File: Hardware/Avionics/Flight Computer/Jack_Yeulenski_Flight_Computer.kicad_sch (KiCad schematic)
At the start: 20 parts, among them J1 SW, J2 BAT, J3 UART Radio Connector, J4 I2C GPS Connector

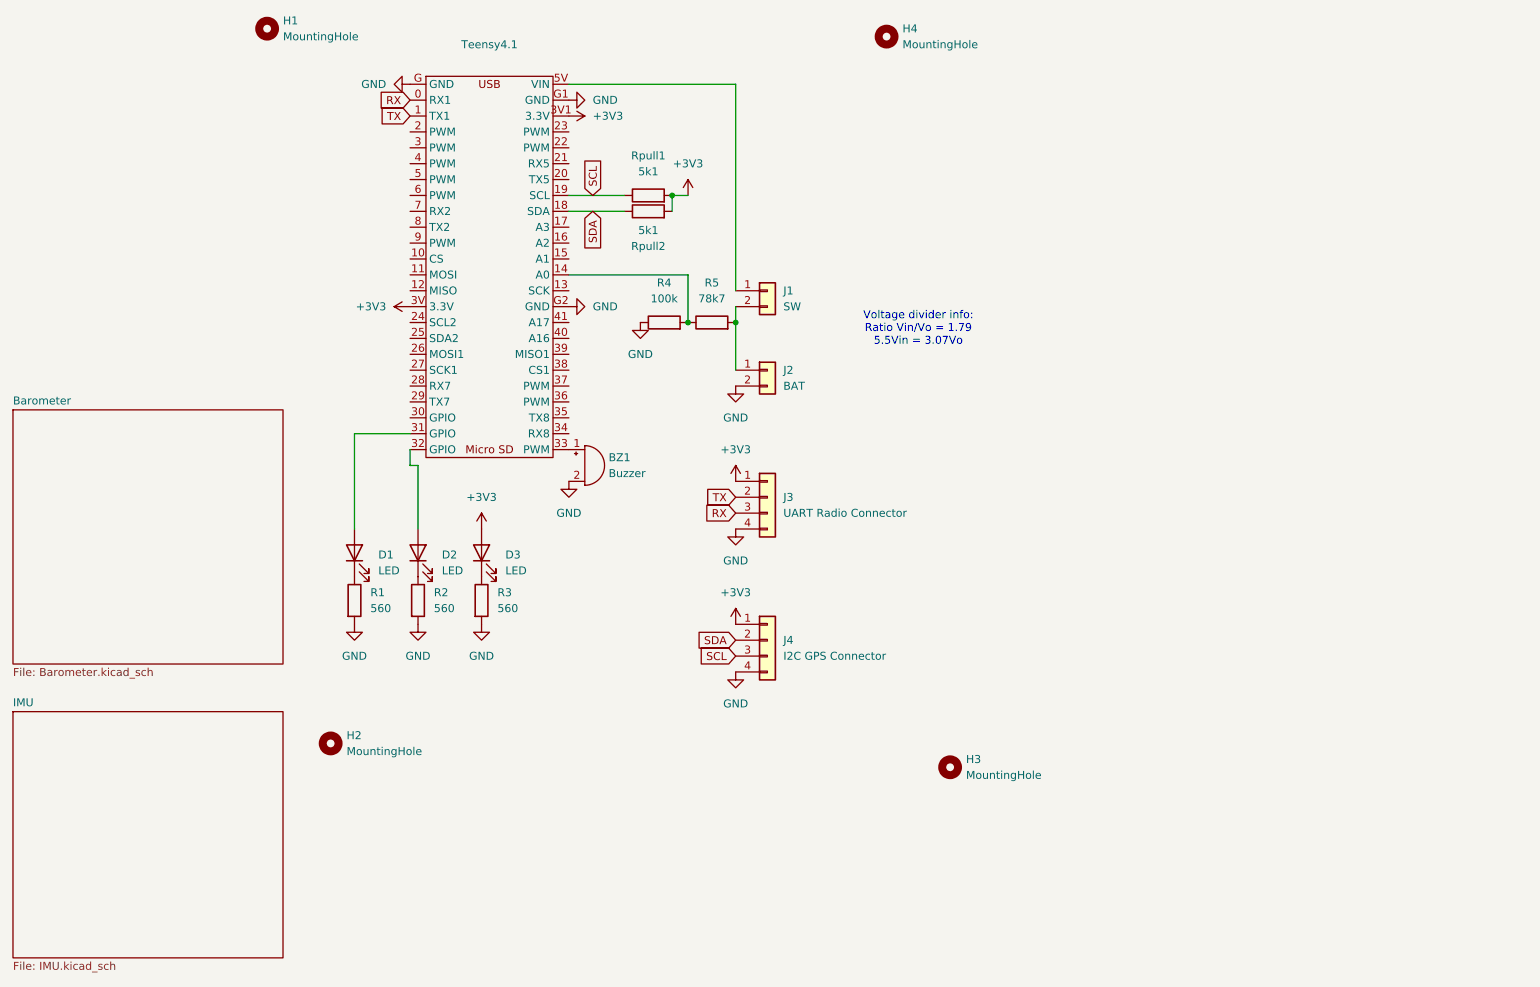
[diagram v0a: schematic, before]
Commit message: PCB updates
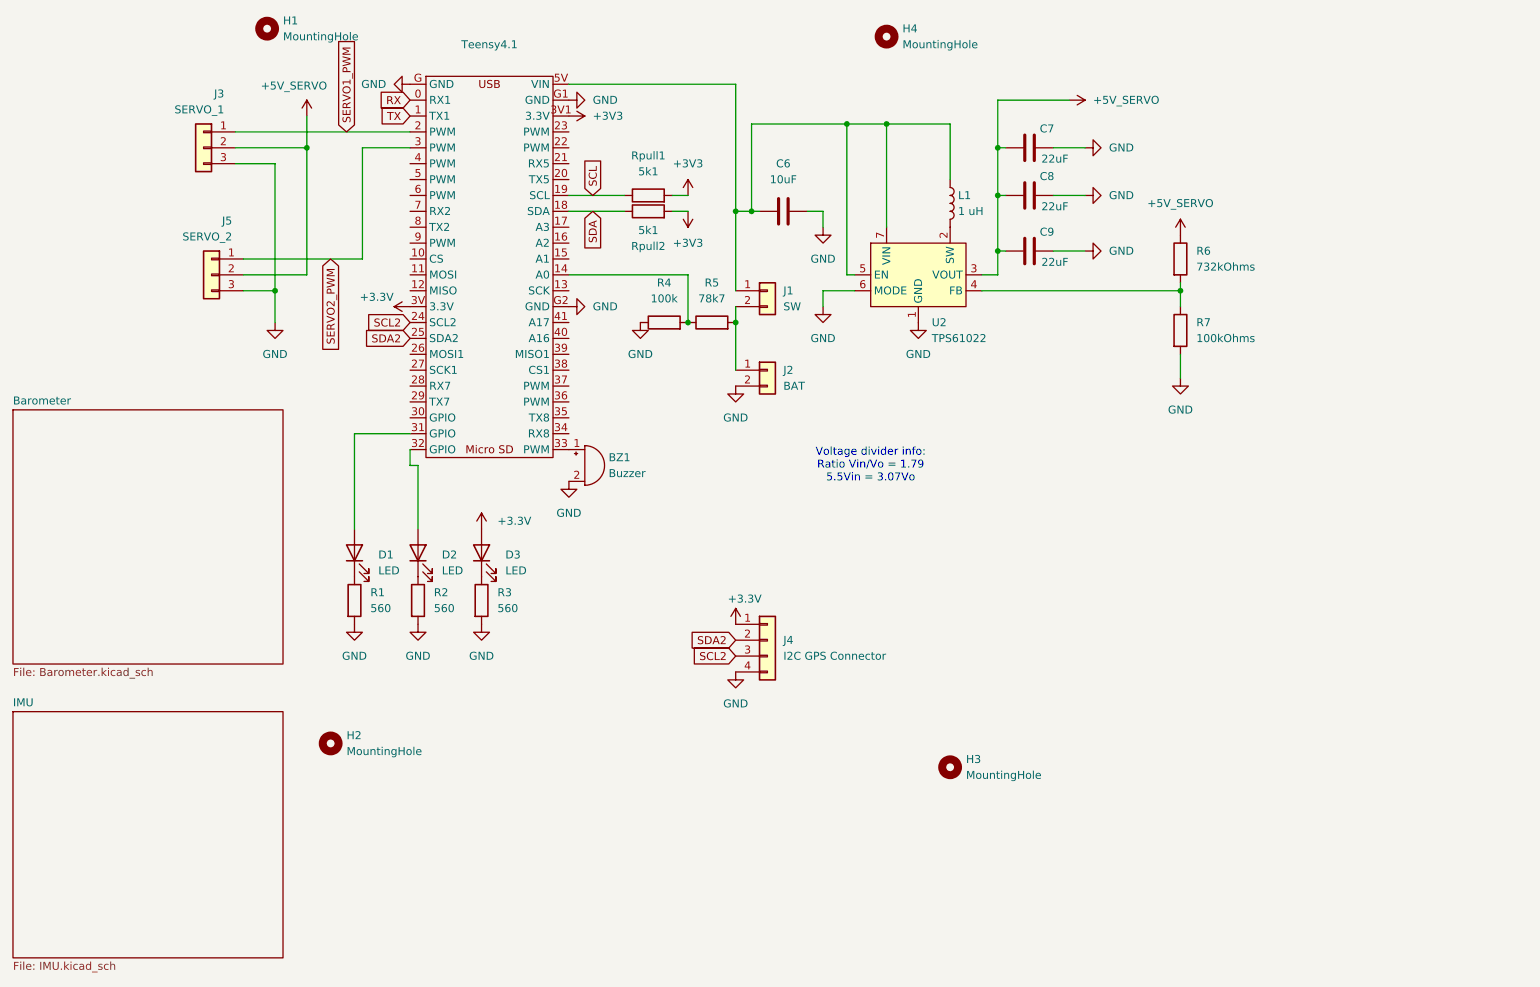
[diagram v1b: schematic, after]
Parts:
- removed J3: UART Radio Connector, Connector_JST:JST_XH_S4B-XH-A_1x04_P2.50mm_Horizontal, symbol Connector_Generic:Conn_01x04
- added C6: 10uF, Capacitor_SMD:C_0805_2012Metric, symbol Device:C
- added C7, C8, C9: 22uF, Capacitor_SMD:C_0805_2012Metric, symbol Device:C
- added J3: SERVO_1, Connector_PinHeader_2.54mm:PinHeader_1x03_P2.54mm_Vertical, symbol Connector_Generic:Conn_01x03
- added J5: SERVO_2, Connector_PinHeader_2.54mm:PinHeader_1x03_P2.54mm_Vertical, symbol Connector_Generic:Conn_01x03
- added L1: 1 uH, Inductor_SMD:L_Coilcraft_XAL7030-102, symbol Device:L
- added R6: 732kOhms, Resistor_SMD:R_0603_1608Metric, symbol Device:R
- added R7: 100kOhms, Resistor_SMD:R_0603_1608Metric, symbol Device:R
- added U2: TPS61022, Package_DFN_QFN:Texas_RWU0007A_VQFN-7_2x2mm_P0.5mm, symbol Converter_DCDC:TPS61022
- Teensy4.1: value ~ -> (none)
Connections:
- net +3V3: no longer D3.2 (A), J4.1 (Pin_1), Teensy4.1.3V (3.3V)
- net GND: now also C6.2, C7.2, C8.2, C9.2, J3.3 (GND), J5.3 (GND), R7.2, U2.1 (GND), U2.6 (MODE)
- net SCL: no longer J4.3 (Pin_3)
- net SDA: no longer J4.2 (Pin_2)
- net SERVO1_PWM: now reaches Teensy4.1.2 (PWM)
- net SERVO1_PWM: now also J3.1 (SERVO_PWM)
- net SCL2: now reaches Teensy4.1.24 (SCL2)
- net SCL2: now also J4.3 (Pin_3)
- net SDA2: now reaches Teensy4.1.25 (SDA2)
- net SDA2: now also J4.2 (Pin_2)
- net SERVO2_PWM: now reaches Teensy4.1.3 (PWM)
- net SERVO2_PWM: now also J5.1 (SERVO_PWM)
- net at J1.1 (Pin_1), Teensy4.1.5V (VIN): now also C6.1, L1.1, U2.5 (EN), U2.7 (VIN)
- new net: L1.2, U2.2 (SW)
- new net: R6.2, R7.1, U2.4 (FB)
- new net +3.3V: D3.2 (A), J4.1 (Pin_1), Teensy4.1.3V (3.3V)
- new net +5V_SERVO: C7.1, C8.1, C9.1, J3.2 (+5V), J5.2 (+5V), R6.1, U2.3 (VOUT)

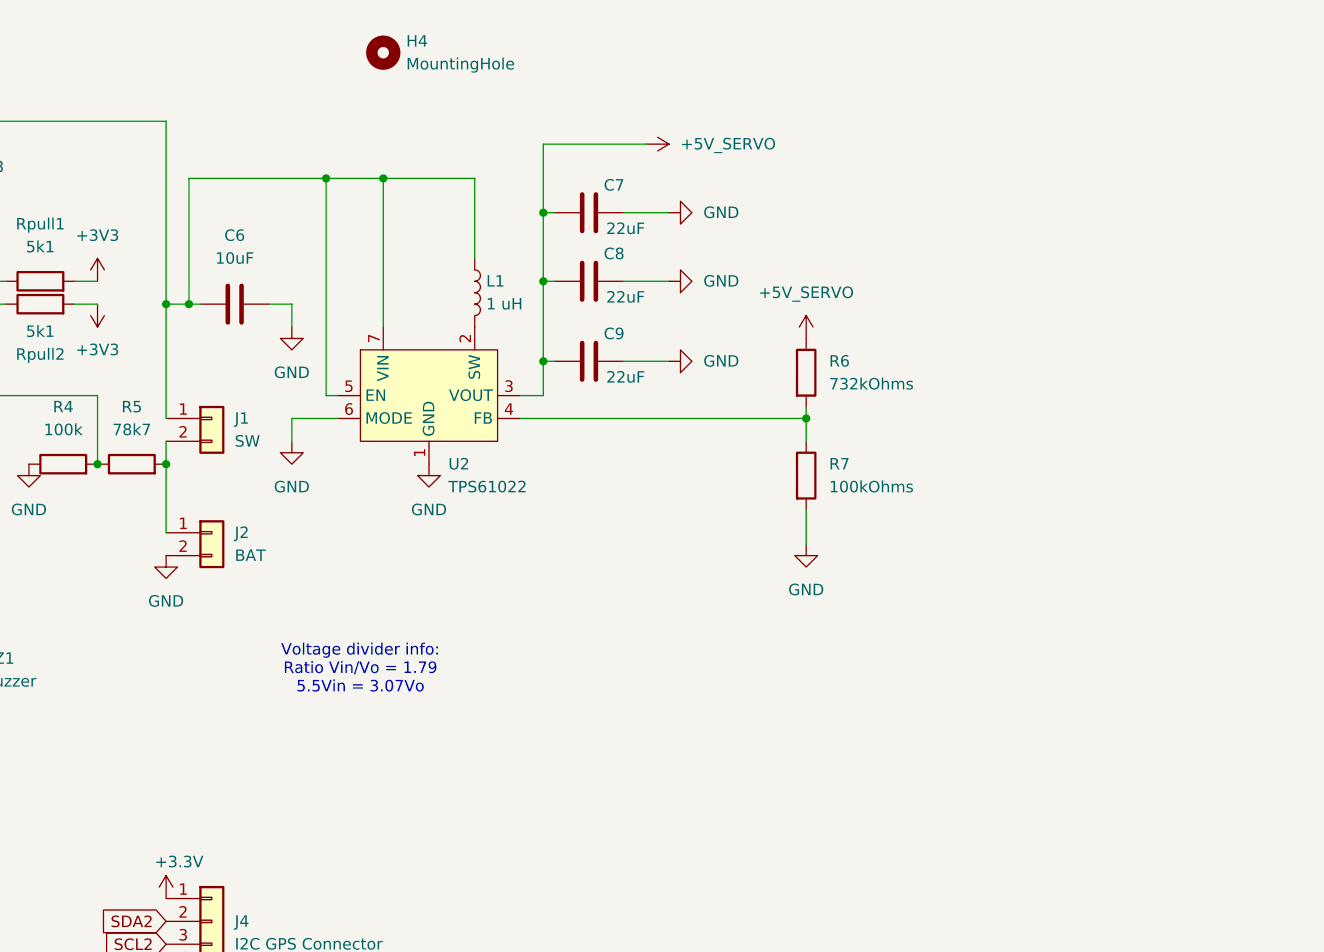
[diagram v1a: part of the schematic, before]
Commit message: updated FC
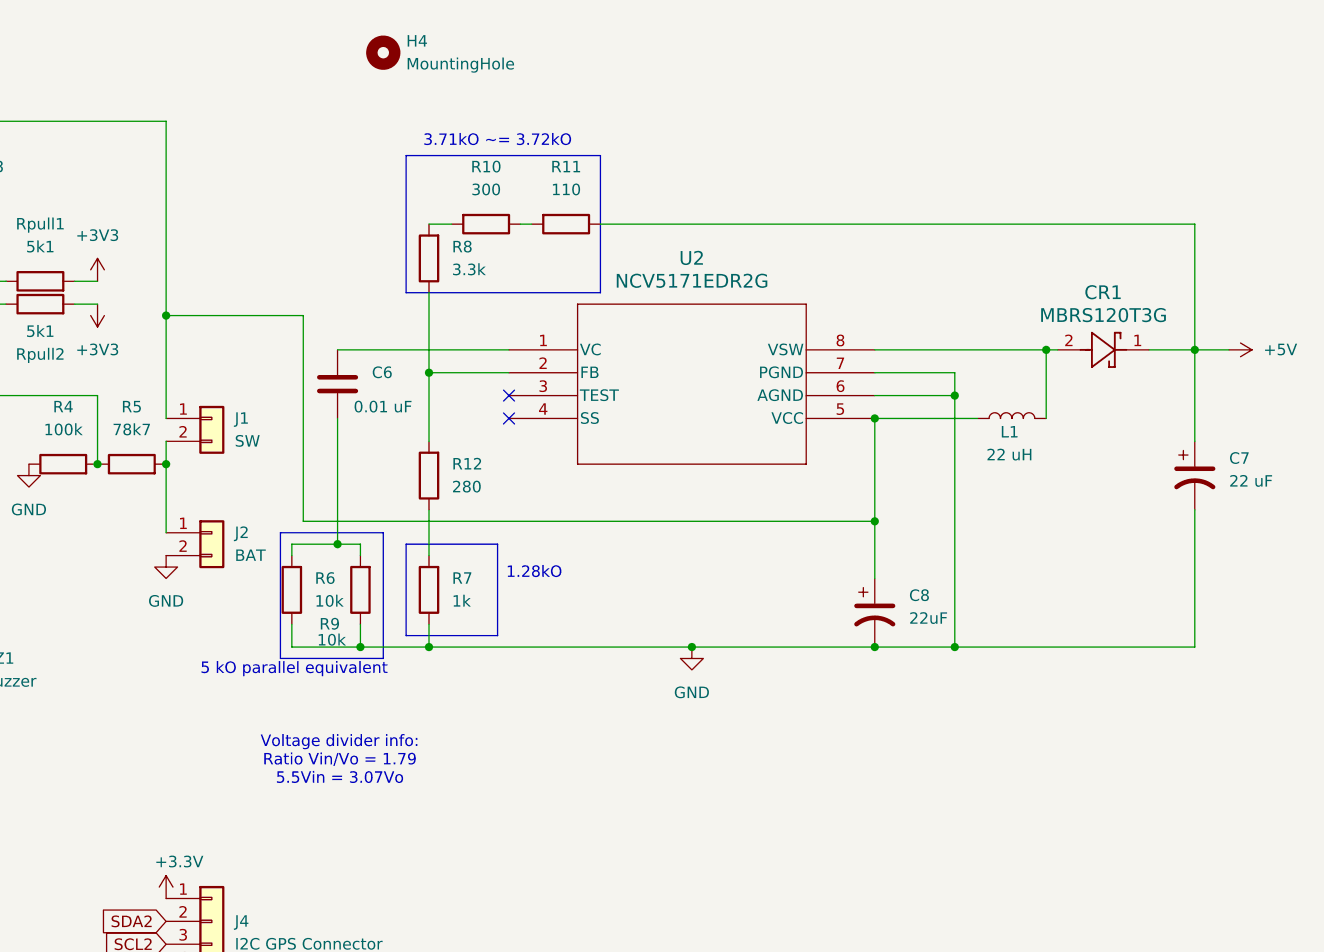
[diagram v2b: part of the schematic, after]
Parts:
- removed C7, C8, C9: 22uF, Capacitor_SMD:C_0805_2012Metric, symbol Device:C
- removed U2: TPS61022, Package_DFN_QFN:Texas_RWU0007A_VQFN-7_2x2mm_P0.5mm, symbol Converter_DCDC:TPS61022
- added C7: 22 uF, Capacitor_SMD:C_0805_2012Metric, symbol Device:C_Polarized_US
- added C8: 22uF, Capacitor_SMD:C_0805_2012Metric, symbol Device:C_Polarized_US
- added CR1: MBRS120T3G, footprints:SDO_MBRS120T3G_OSI, symbol 2026-09-30_23-48-21:MBRS120T3G
- added R10: 300, Resistor_SMD:R_0603_1608Metric, symbol Device:R
- added R11: 110, Resistor_SMD:R_0603_1608Metric, symbol Device:R
- added R12: 280, Resistor_SMD:R_0603_1608Metric, symbol Device:R
- added R8: 3.3k, Resistor_SMD:R_0603_1608Metric, symbol Device:R
- added R9: 10k, Resistor_SMD:R_0603_1608Metric, symbol Device:R
- added U2: NCV5171EDR2G, footprints:SOIC-8_NB_ONS, symbol 2026-09-30_15-53-03:NCV5171EDR2G
- C6: value 10uF -> 0.01 uF
- J3, J5: footprint Connector_PinHeader_2.54mm:PinHeader_1x03_P2.54mm_Vertical -> Connector_JST:JST_XH_S3B-XH-A-1_1x03_P2.50mm_Horizontal
- L1: value 1 uH -> 22 uH
- R6: value 732kOhms -> 10k
- R7: value 100kOhms -> 1k
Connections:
- net +5V_SERVO: no longer R6.1
- net GND: now also R6.1, R7.1, C7.2, C8.2, R9.1, U2.6 (AGND), U2.7 (PGND); no longer C6.2, R7.2
- net at J1.1 (Pin_1), L1.1, Teensy4.1.5V (VIN): now also C8.1, U2.5 (VCC); no longer C6.1
- net at L1.2: now also CR1.2, U2.8 (VSW)
- net at R6.2: now also C6.2, R9.2; no longer R7.1
- new net: C6.1, U2.1 (VC)
- new net: R12.1, R7.2
- new net: R12.2, R8.1, U2.2 (FB)
- new net: R10.1, R11.2
- new net: R10.2, R8.2
- new net +5V: C7.1, CR1.1, R11.1
- no-connect marks 0 -> 2
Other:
- note added: "1.28kO"
- note added: "3.71kO ~= 3.72kO"
- note added: "5 kO parallel equivalent"
- moved on the sheet: L1
